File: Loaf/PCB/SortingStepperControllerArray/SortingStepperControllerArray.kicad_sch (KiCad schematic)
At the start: 26 parts, among them J1 Conn_01x04_Socket, J2 Conn_01x04_Socket, J3 Conn_01x04_Socket, J4 Conn_01x04_Socket, J5 Motor_Supply, J6 Logic_Supply, J7 Logic_Input, SW1 Limit_Switch, SW2 Limit_Switch, SW3 Limit_Switch, SW4 Limit_Switch

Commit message: Reoriented board for less signal interference
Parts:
- C1, C2, C3, C4: footprint Capacitor_THT:C_Rect_L7.0mm_W2.0mm_P5.00mm -> Capacitor_THT:CP_Radial_D8.0mm_P3.50mm
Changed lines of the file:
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@@
 			)
 		)
-		(property "Footprint" "Capacitor_THT:C_Rect_L7.0mm_W2.0mm_P5.00mm"
+		(property "Footprint" "Capacitor_THT:CP_Radial_D8.0mm_P3.50mm"
 			(at 229.87 20.6248 0)
 			(hide yes)
@@
 			)
 		)
-		(property "Footprint" "Capacitor_THT:C_Rect_L7.0mm_W2.0mm_P5.00mm"
+		(property "Footprint" "Capacitor_THT:CP_Radial_D8.0mm_P3.50mm"
 			(at 96.52 20.6248 0)
 			(hide yes)
@@
 			)
 		)
-		(property "Footprint" "Capacitor_THT:C_Rect_L7.0mm_W2.0mm_P5.00mm"
+		(property "Footprint" "Capacitor_THT:CP_Radial_D8.0mm_P3.50mm"
 			(at 185.42 20.6248 0)
 			(hide yes)
@@
 			)
 		)
-		(property "Footprint" "Capacitor_THT:C_Rect_L7.0mm_W2.0mm_P5.00mm"
+		(property "Footprint" "Capacitor_THT:CP_Radial_D8.0mm_P3.50mm"
 			(at 140.97 20.6248 0)
 			(hide yes)

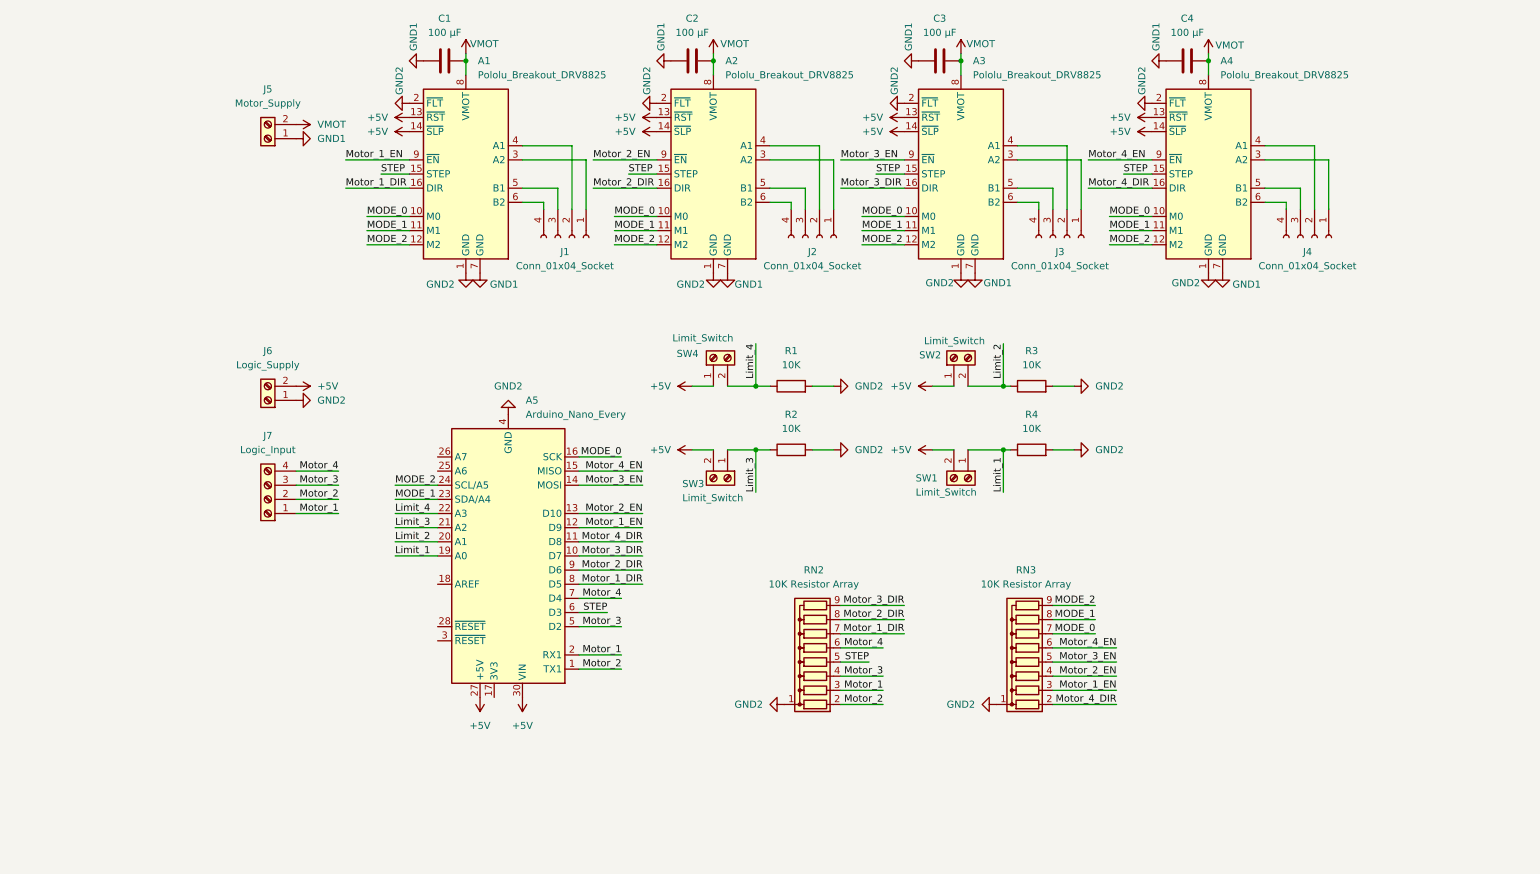
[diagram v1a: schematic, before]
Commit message: Redid the stepper board
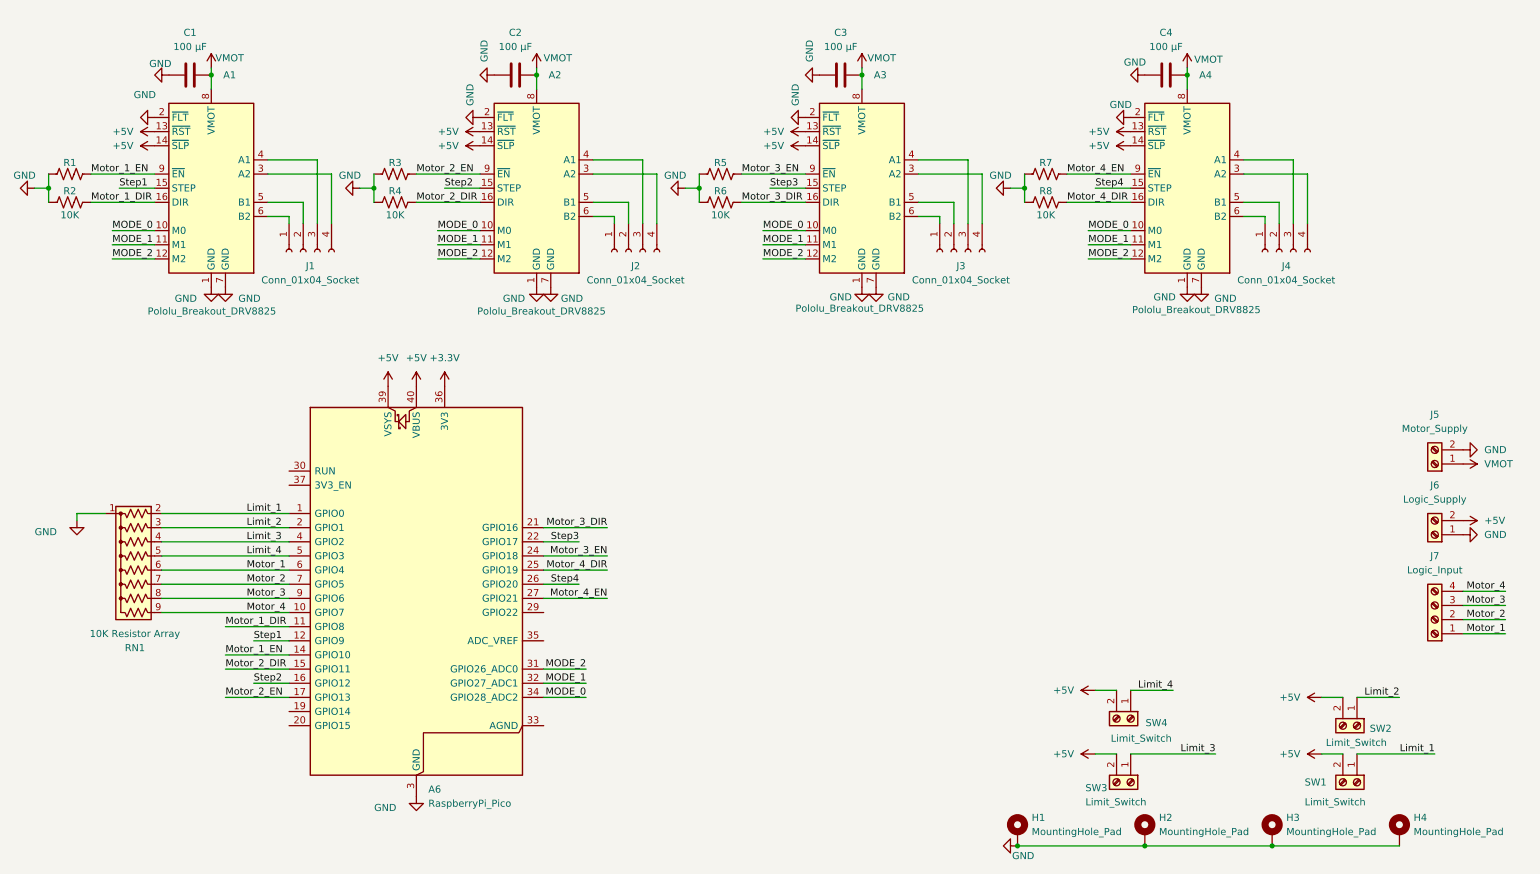
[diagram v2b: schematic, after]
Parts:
- removed A5: Arduino_Nano_Every, Module:Arduino_Nano, symbol MCU_Module:Arduino_Nano_Every
- removed R1, R2, R3, R4: 10K, Resistor_THT:R_Axial_DIN0204_L3.6mm_D1.6mm_P7.62mm_Horizontal, symbol Device:R
- removed RN2, RN3: 10K Resistor Array, Resistor_THT:R_Array_SIP9, symbol Device:R_Network08
- added A6: RaspberryPi_Pico, Module:RaspberryPi_Pico_Common_Unspecified, symbol MCU_Module:RaspberryPi_Pico
- added H1, H2, H3, H4: MountingHole_Pad, MountingHole:MountingHole_3.2mm_M3_DIN965_Pad, symbol Mechanical:MountingHole_Pad
- added R1, R2, R3, R4, R5, R6, R7, R8: 10K, R_1206_3216Metric_Pad1.30x1.75mm_HandSolder, symbol Device:R_US
- added RN1: 10K Resistor Array, Resistor_THT:R_Array_SIP9, symbol Device:R_Network08_US
- J1, J2, J3, J4: footprint Connector_JST:JST_PH_B4B-PH-K_1x04_P2.00mm_Vertical -> JST_XH_B4B-XH-A_1x04_P2.50mm_Vertical
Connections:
- net GND2 is gone; now on net GND: A1.1 (GND), A1.2 (~{FLT}), A2.1 (GND), A2.2 (~{FLT}), A3.1 (GND), A3.2 (~{FLT}), A4.1 (GND), A4.2 (~{FLT}), J6.1 (Pin_1)
- net +5V: now also SW2.2 (Pin_2), SW4.2 (Pin_2), A6.39 (VSYS), A6.40 (VBUS); no longer SW2.1 (Pin_1), SW4.1 (Pin_1)
- net Limit_1: now also A6.1 (GPIO0), RN1.2 (R1)
- net Limit_2: now also SW2.1 (Pin_1), A6.2 (GPIO1), RN1.3 (R2); no longer SW2.2 (Pin_2)
- net Limit_3: now also A6.4 (GPIO2), RN1.4 (R3)
- net Limit_4: now also SW4.1 (Pin_1), A6.5 (GPIO3), RN1.5 (R4); no longer SW4.2 (Pin_2)
- net MODE_0: now also A6.34 (GPIO28_ADC2)
- net MODE_1: now also A6.32 (GPIO27_ADC1)
- net MODE_2: now also A6.31 (GPIO26_ADC0)
- net Motor_1: now also A6.6 (GPIO4), RN1.6 (R5)
- net Motor_1_DIR: now also A6.11 (GPIO8), R2.2
- net Motor_1_EN: now also A6.14 (GPIO10), R1.2
- net Motor_2: now also A6.7 (GPIO5), RN1.7 (R6)
- net Motor_2_DIR: now also A6.15 (GPIO11), R4.2
- net Motor_2_EN: now also A6.17 (GPIO13), R3.2
- net Motor_3: now also A6.9 (GPIO6), RN1.8 (R7)
- net Motor_3_DIR: now also A6.21 (GPIO16), R6.2
- net Motor_3_EN: now also A6.24 (GPIO18), R5.2
- net Motor_4: now also A6.10 (GPIO7), RN1.9 (R8)
- net Motor_4_DIR: now also A6.25 (GPIO19), R8.2
- net Motor_4_EN: now also A6.27 (GPIO21), R7.2
- net VMOT: now also J5.1 (Pin_1); no longer J5.2 (Pin_2)
- net at A3.3 (A2): now also J3.4 (Pin_4); no longer J3.1 (Pin_1)
- net at A3.4 (A1): now also J3.3 (Pin_3); no longer J3.2 (Pin_2)
- net at A3.5 (B1): now also J3.2 (Pin_2); no longer J3.3 (Pin_3)
- net at A3.6 (B2): now also J3.1 (Pin_1); no longer J3.4 (Pin_4)
- net at J2.1 (Pin_1): now also A2.6 (B2); no longer A2.3 (A2)
- net at J2.2 (Pin_2): now also A2.5 (B1); no longer A2.4 (A1)
- net at J2.3 (Pin_3): now also A2.4 (A1); no longer A2.5 (B1)
- net at J2.4 (Pin_4): now also A2.3 (A2); no longer A2.6 (B2)
- net at J1.1 (Pin_1): now also A1.6 (B2); no longer A1.3 (A2)
- net at J1.2 (Pin_2): now also A1.5 (B1); no longer A1.4 (A1)
- net at J1.3 (Pin_3): now also A1.4 (A1); no longer A1.5 (B1)
- net at J1.4 (Pin_4): now also A1.3 (A2); no longer A1.6 (B2)
- net at J4.1 (Pin_1): now also A4.6 (B2); no longer A4.3 (A2)
- net at J4.2 (Pin_2): now also A4.5 (B1); no longer A4.4 (A1)
- net at J4.3 (Pin_3): now also A4.4 (A1); no longer A4.5 (B1)
- net at J4.4 (Pin_4): now also A4.3 (A2); no longer A4.6 (B2)
- net GND1 renamed GND
- net GND: now also J5.2 (Pin_2), A6.13 (GND), A6.18 (GND), A6.23 (GND), A6.28 (GND), A6.3 (GND), A6.38 (GND), A6.8 (GND), H1.1, H2.1, H3.1, H4.1, R1.1, R2.1, R3.1, R4.1, R5.1, R6.1, R7.1, R8.1, RN1.1 (common); no longer J5.1 (Pin_1)
- removed net STEP: A1.15 (STEP), A2.15 (STEP), A3.15 (STEP), A4.15 (STEP)
- new net +3.3V: A6.36 (3V3)
- new net Step1: A1.15 (STEP), A6.12 (GPIO9)
- new net Step2: A2.15 (STEP), A6.16 (GPIO12)
- new net Step3: A3.15 (STEP), A6.22 (GPIO17)
- new net Step4: A4.15 (STEP), A6.26 (GPIO20)
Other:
- moved on the sheet: A1, A2, A3, A4, C1, C2, C3, C4, J6, J7, SW1, SW3

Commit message: Updated control board footprints
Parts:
- J5, J6, SW1, SW2, SW3, SW4: footprint TerminalBlock:TerminalBlock_Xinya_XY308-2.54-2P_1x02_P2.54mm_Horizontal -> TerminalBlock_TE-Connectivity:TerminalBlock_TE_282834-2_1x02_P2.54mm_Horizontal
- J7: footprint TerminalBlock:TerminalBlock_Xinya_XY308-2.54-4P_1x04_P2.54mm_Horizontal -> TerminalBlock_TE-Connectivity:TerminalBlock_TE_282834-4_1x04_P2.54mm_Horizontal
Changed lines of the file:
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@@
 			)
 		)
-		(property "Footprint" "TerminalBlock:TerminalBlock_Xinya_XY308-2.54-2P_1x02_P2.54mm_Horizontal"
+		(property "Footprint" "TerminalBlock_TE-Connectivity:TerminalBlock_TE_282834-2_1x02_P2.54mm_Horizontal"
 			(at 256.54 140.97 0)
 			(hide yes)
@@
 			)
 		)
-		(property "Footprint" "TerminalBlock:TerminalBlock_Xinya_XY308-2.54-2P_1x02_P2.54mm_Horizontal"
+		(property "Footprint" "TerminalBlock_TE-Connectivity:TerminalBlock_TE_282834-2_1x02_P2.54mm_Horizontal"
 			(at 215.9 139.7 0)
 			(hide yes)
@@
 			)
 		)
-		(property "Footprint" "TerminalBlock:TerminalBlock_Xinya_XY308-2.54-2P_1x02_P2.54mm_Horizontal"
+		(property "Footprint" "TerminalBlock_TE-Connectivity:TerminalBlock_TE_282834-2_1x02_P2.54mm_Horizontal"
 			(at 270.51 93.98 0)
 			(hide yes)
@@
 			)
 		)
-		(property "Footprint" "TerminalBlock:TerminalBlock_Xinya_XY308-2.54-4P_1x04_P2.54mm_Horizontal"
+		(property "Footprint" "TerminalBlock_TE-Connectivity:TerminalBlock_TE_282834-4_1x04_P2.54mm_Horizontal"
 			(at 270.51 121.92 0)
 			(hide yes)
@@
 			)
 		)
-		(property "Footprint" "TerminalBlock:TerminalBlock_Xinya_XY308-2.54-2P_1x02_P2.54mm_Horizontal"
+		(property "Footprint" "TerminalBlock_TE-Connectivity:TerminalBlock_TE_282834-2_1x02_P2.54mm_Horizontal"
 			(at 256.54 151.13 0)
 			(hide yes)
@@
 			)
 		)
-		(property "Footprint" "TerminalBlock:TerminalBlock_Xinya_XY308-2.54-2P_1x02_P2.54mm_Horizontal"
+		(property "Footprint" "TerminalBlock_TE-Connectivity:TerminalBlock_TE_282834-2_1x02_P2.54mm_Horizontal"
 			(at 270.51 106.68 0)
 			(hide yes)
@@
 			)
 		)
-		(property "Footprint" "TerminalBlock:TerminalBlock_Xinya_XY308-2.54-2P_1x02_P2.54mm_Horizontal"
+		(property "Footprint" "TerminalBlock_TE-Connectivity:TerminalBlock_TE_282834-2_1x02_P2.54mm_Horizontal"
 			(at 215.9 151.13 0)
 			(hide yes)
